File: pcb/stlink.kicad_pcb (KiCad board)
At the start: 4 copper layers, 42 x 26 mm, 41 parts, among them J1 USB_A, Q1 S9013, U1 XC6206P332MR, U2 STM32F103CB, Y1 8MHz

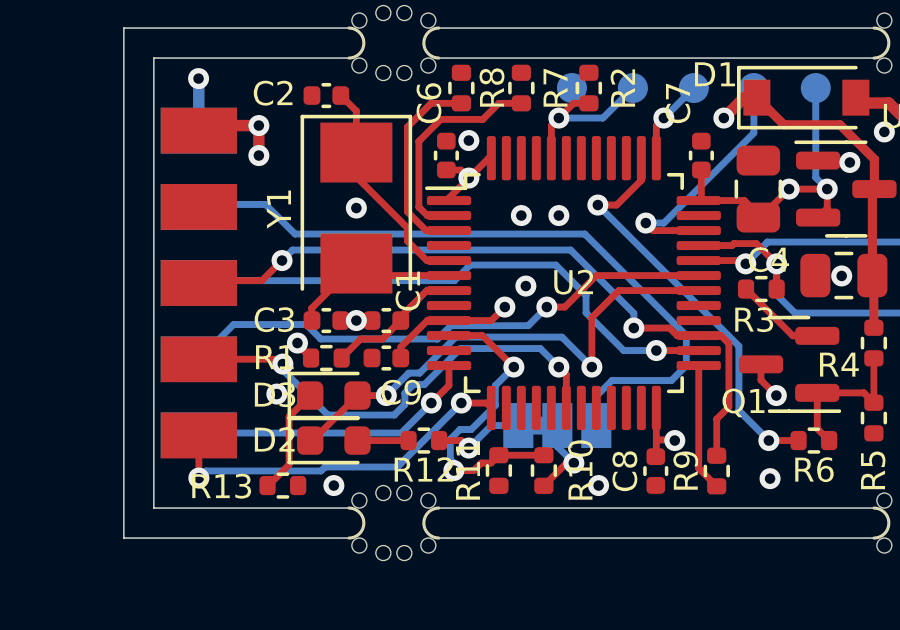
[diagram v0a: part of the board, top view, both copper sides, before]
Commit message: Hmmmm
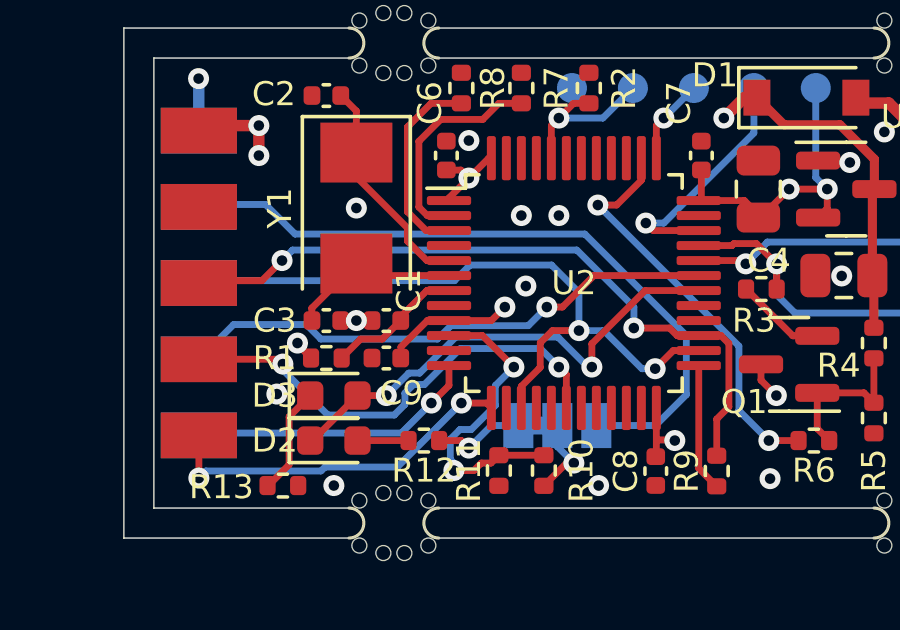
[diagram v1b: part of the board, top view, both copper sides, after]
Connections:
- U2 pad 15: unconnected-(U2-Pad15) -> T_CLK
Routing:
- net T_CLK: track 18.3 -> 23.1 mm, vias 1 -> 2
- net LED: track 16.7 -> 16.2 mm
